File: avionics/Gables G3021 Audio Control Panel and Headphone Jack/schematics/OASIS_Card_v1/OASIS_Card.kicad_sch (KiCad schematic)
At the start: 57 parts, among them J1 Conn_02x08_Top_Bottom, J3 12v DC, J4 AudioJack3_Ground_Switch, J5 Control Signals Out, J6 12v DC OUT, J7 Piggyback Master, J8 Piggyback Slave, J9 12v DC, U1 CD4051B, U3 LTC1044

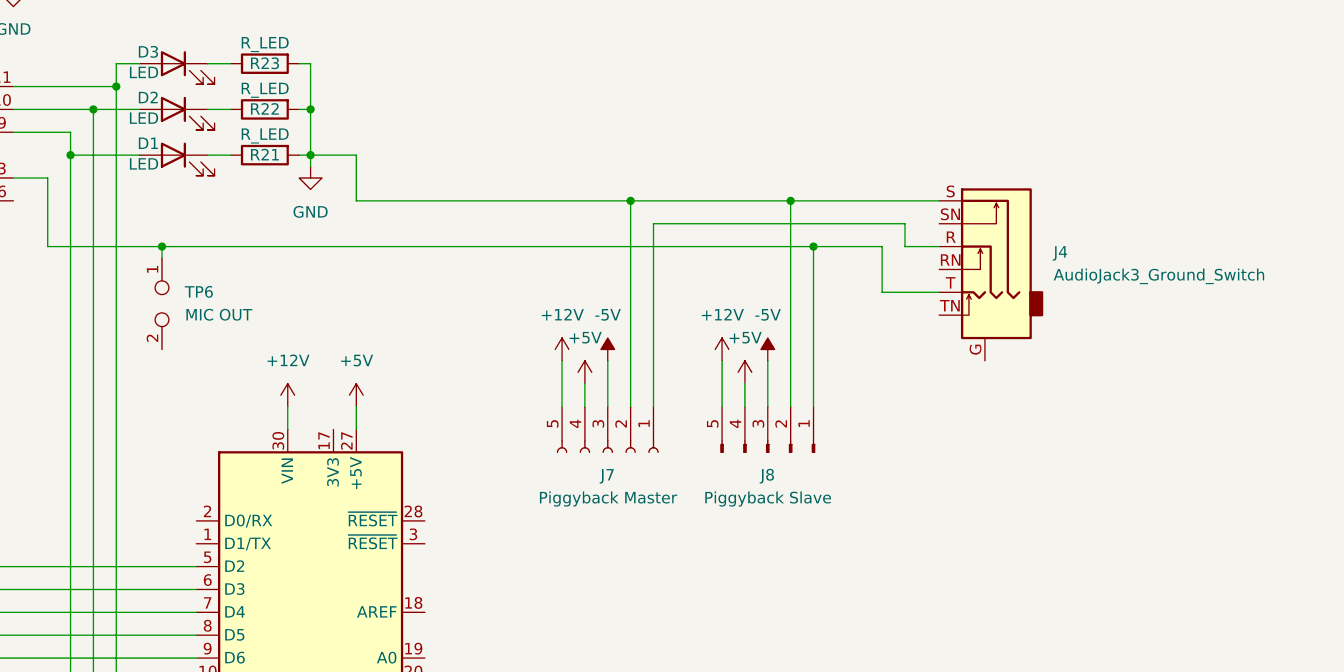
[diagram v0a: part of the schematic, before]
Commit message: more OASIS card stuff
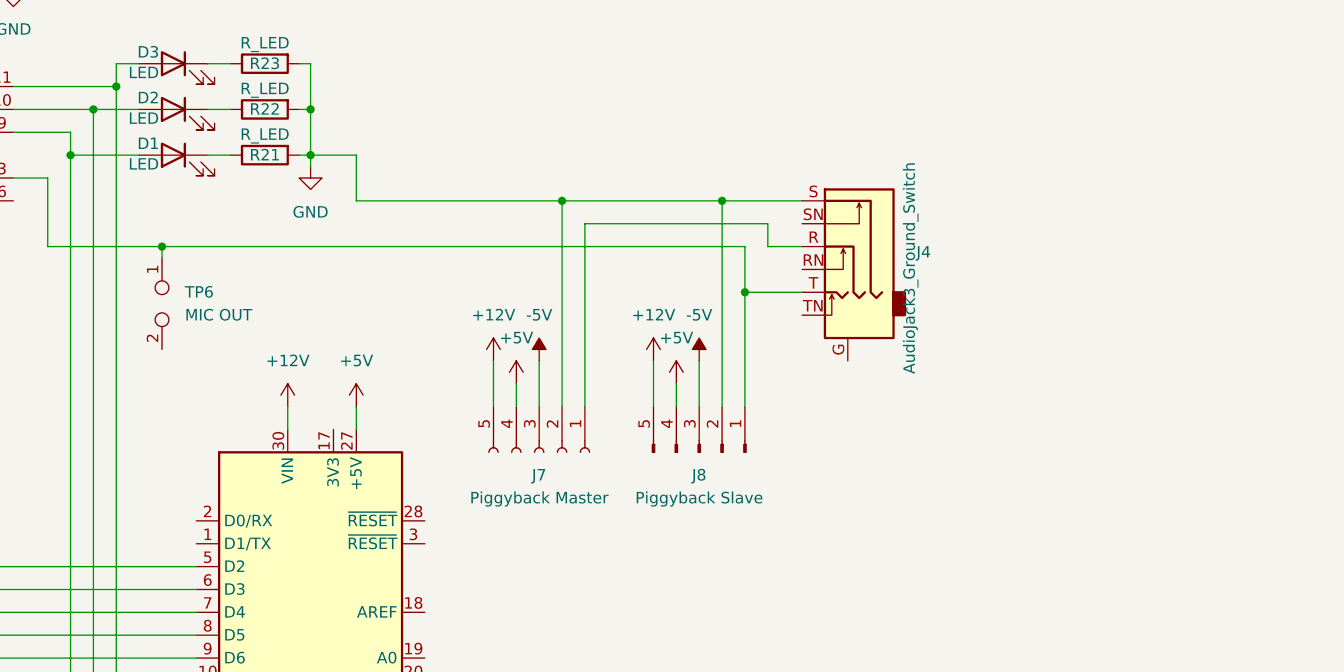
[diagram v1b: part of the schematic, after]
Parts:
- TP2, TP3, TP4: footprint Connector_PinHeader_2.54mm:PinHeader_1x01_P2.54mm_Vertical -> TestPoint:TestPoint_Pad_2.5x2.5mm
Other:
- moved on the sheet: J4, J7, J8
